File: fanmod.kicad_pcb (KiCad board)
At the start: 2 copper layers, 15 x 15 mm, 6 parts, among them J1 FAN_IN, J2 FAN_OUT, J4 COMM

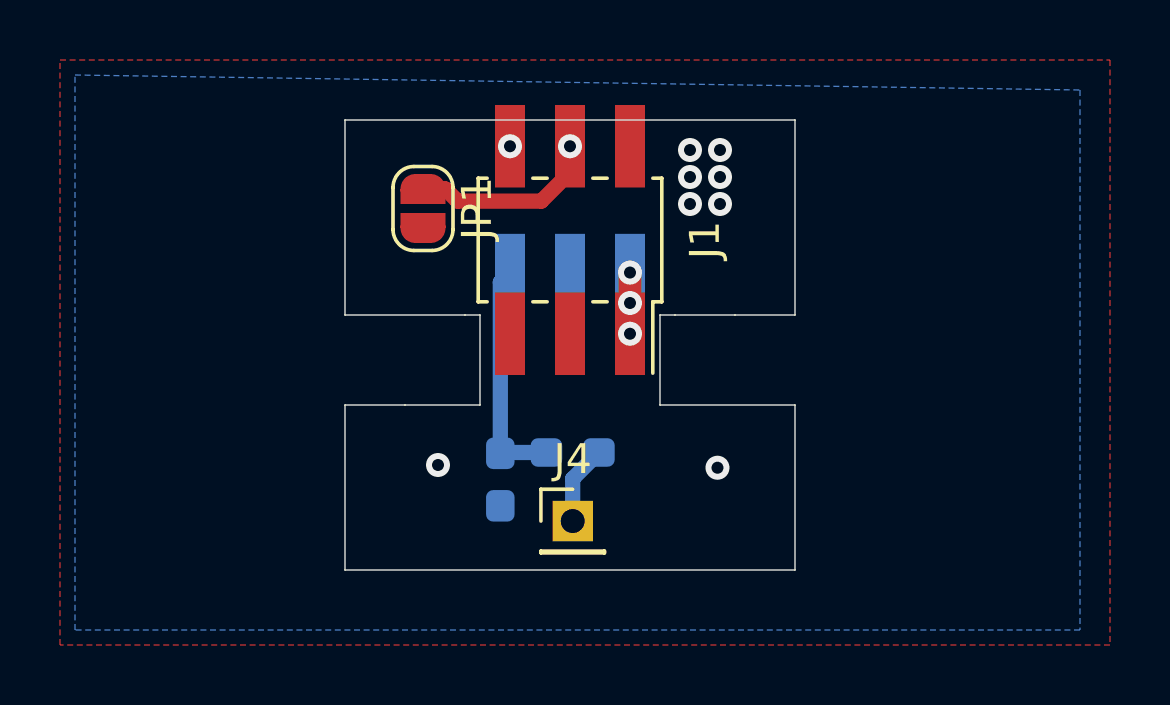
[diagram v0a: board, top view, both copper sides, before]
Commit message: board v2.0
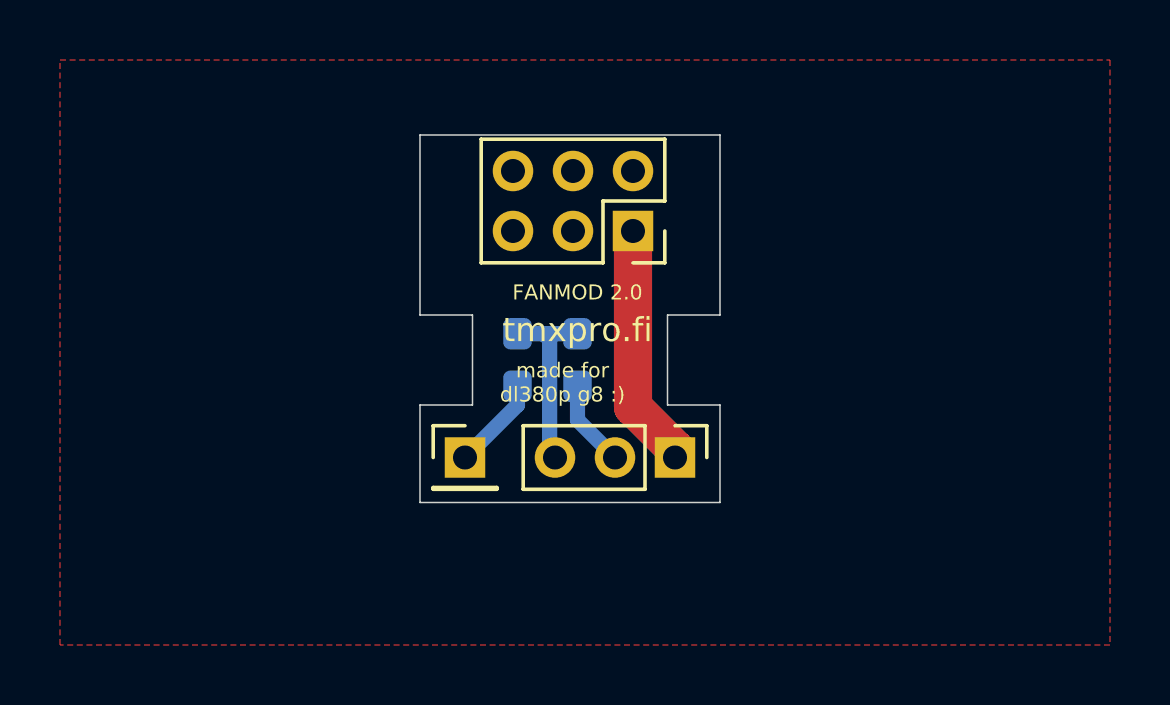
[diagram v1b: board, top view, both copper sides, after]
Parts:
- removed JP1: BYPASS, Jumper:SolderJumper-2_P1.3mm_Open_RoundedPad1.0x1.5mm
- J1: footprint Connector_PinSocket_2.00mm:PinSocket_2x03_P2.00mm_Vertical_SMD -> Connector_PinSocket_2.00mm:PinSocket_2x03_P2.00mm_Vertical
- J2: value FAN_OUT -> HACKY_OUT; footprint Connector_PinHeader_2.00mm:PinHeader_2x03_P2.00mm_Vertical_SMD -> Connector_PinHeader_2.00mm:PinHeader_1x03_P2.00mm_Vertical; moved to F.Cu
- R1: value 1k -> 4.7k
- R2: value 2k -> 10k
- moved J2 8.96 mm to (88.5, 29.2), turned to 270 degrees
- moved R2 4.74 mm to (85.2, 26.0)
- moved J4 4.17 mm to (81.5, 29.2)
- moved R1 3.59 mm to (83.2, 26.0), turned to 90 degrees
- moved J1 2.12 mm to (87.1, 21.7)
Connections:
- J1 pad 4: GROUND_LOOP -> GND
- J1 pad 6: ROTATION_DETECT -> GND
- J2 pad 3: (no net) -> Net-(J2-Pad3)
- R1 pad 2: Net-(J2-Pad5) -> Net-(J2-Pad3)
- R2 pad 1: Net-(J2-Pad5) -> Net-(J2-Pad3)
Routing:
- net +12V: track 4.08 -> 16.3 mm, vias 3 -> 0
- net Net-(J2-Pad5): track 7.71 -> 0.00 mm
- net GROUND_LOOP: track 6.34 -> 0.00 mm, vias 1 -> 0
- net Net-(J2-Pad3): track 0.00 -> 6.28 mm
- net GND: track 0.00 -> 2.89 mm, vias 8 -> 0
- net ROTATION_DETECT: track 0.04 -> 0.00 mm, vias 1 -> 0
- removed copper zone on B.Cu, net GND
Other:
- board size 15 x 15 mm -> 10 x 12.2 mm
- board text added: "FANMOD 2.0"
- board text added: "made for dl380p g8 :)"
- board text added: "tmxpro.fi"
